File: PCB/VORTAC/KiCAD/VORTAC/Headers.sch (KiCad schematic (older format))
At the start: 15 parts, among them J1 MillMax_004, J10 HEATER, J11 STEPPER, J12 IO, J13 918-418K2023S40001, J2 MillMax_004, J3 DOCK, J4 USB_HOST, J5 FAN_01, J6 FAN_02, J7 LED, J8 HOTEND, J9 THERM

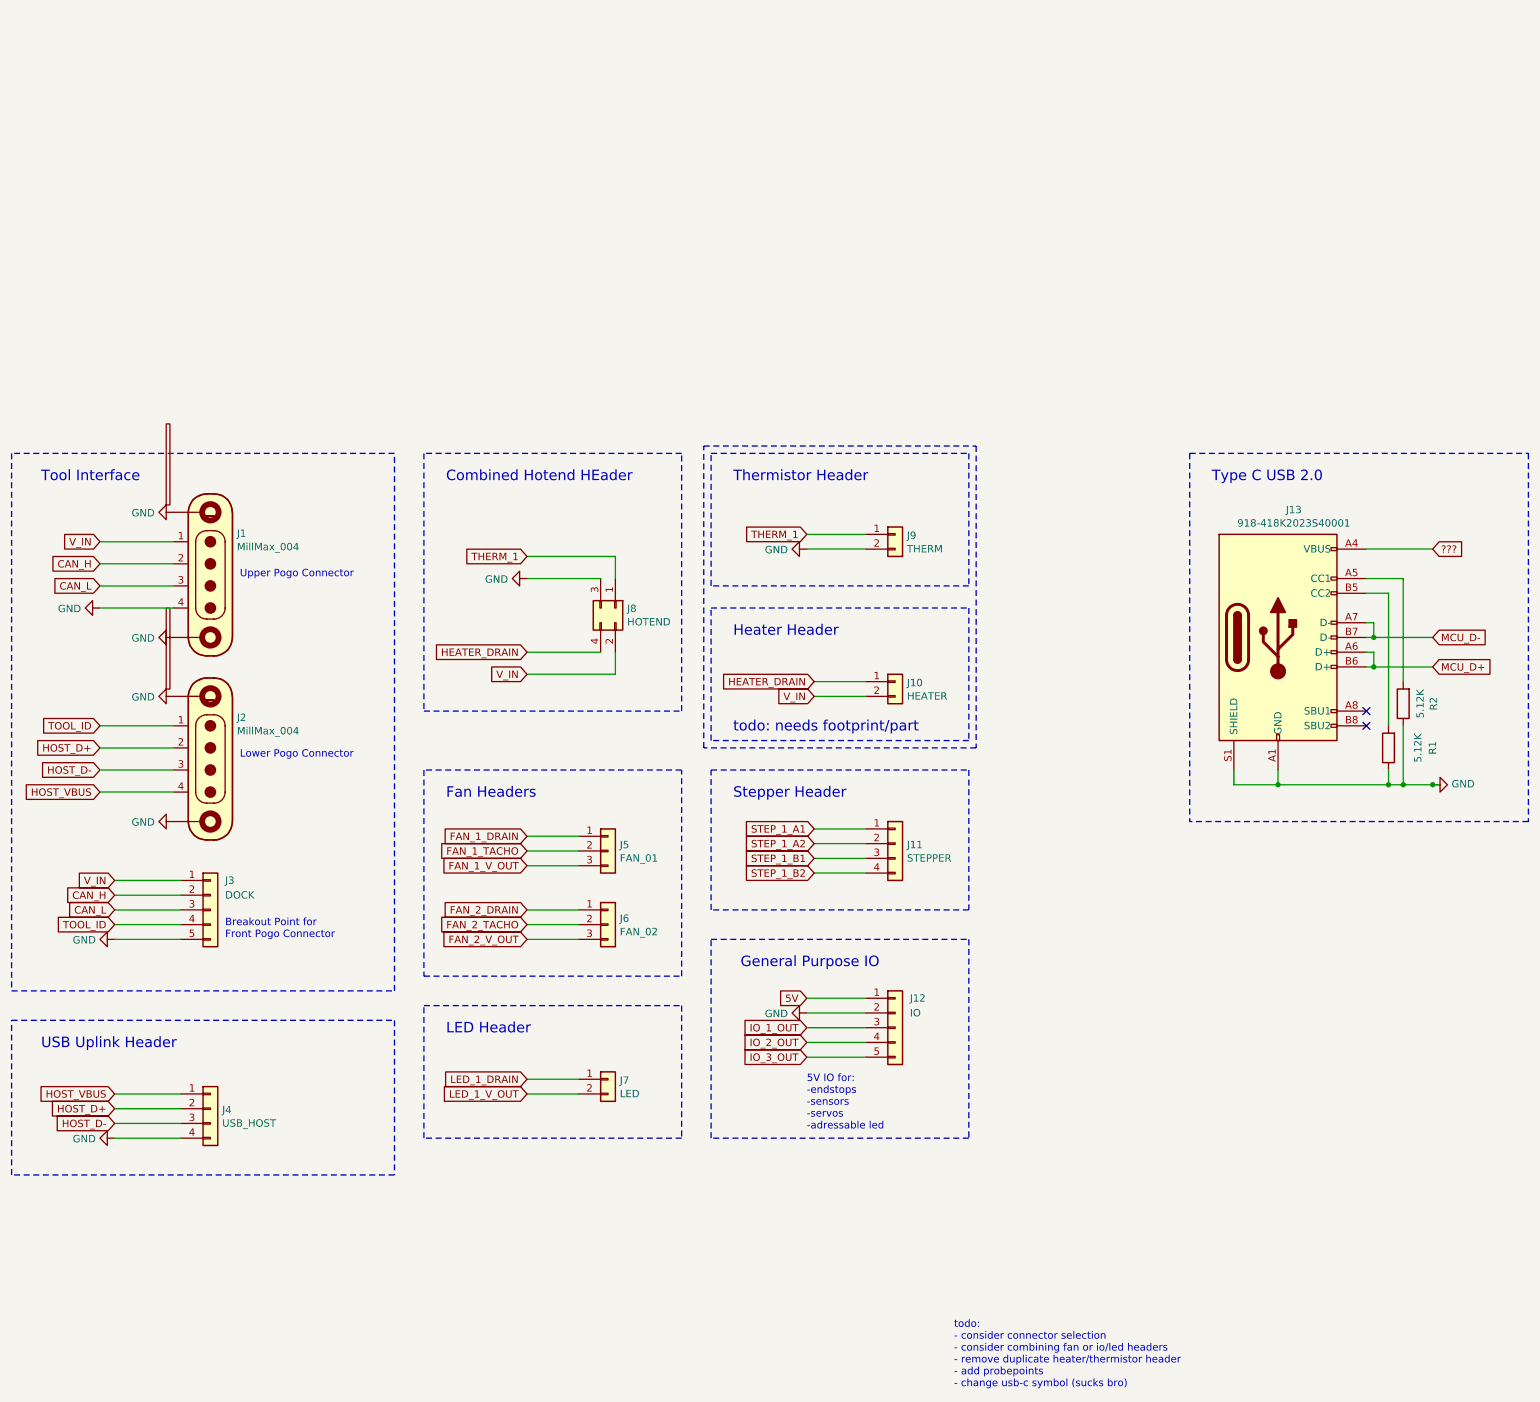
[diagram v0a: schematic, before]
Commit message: Auto stash before merge of "main" and "origin/main"
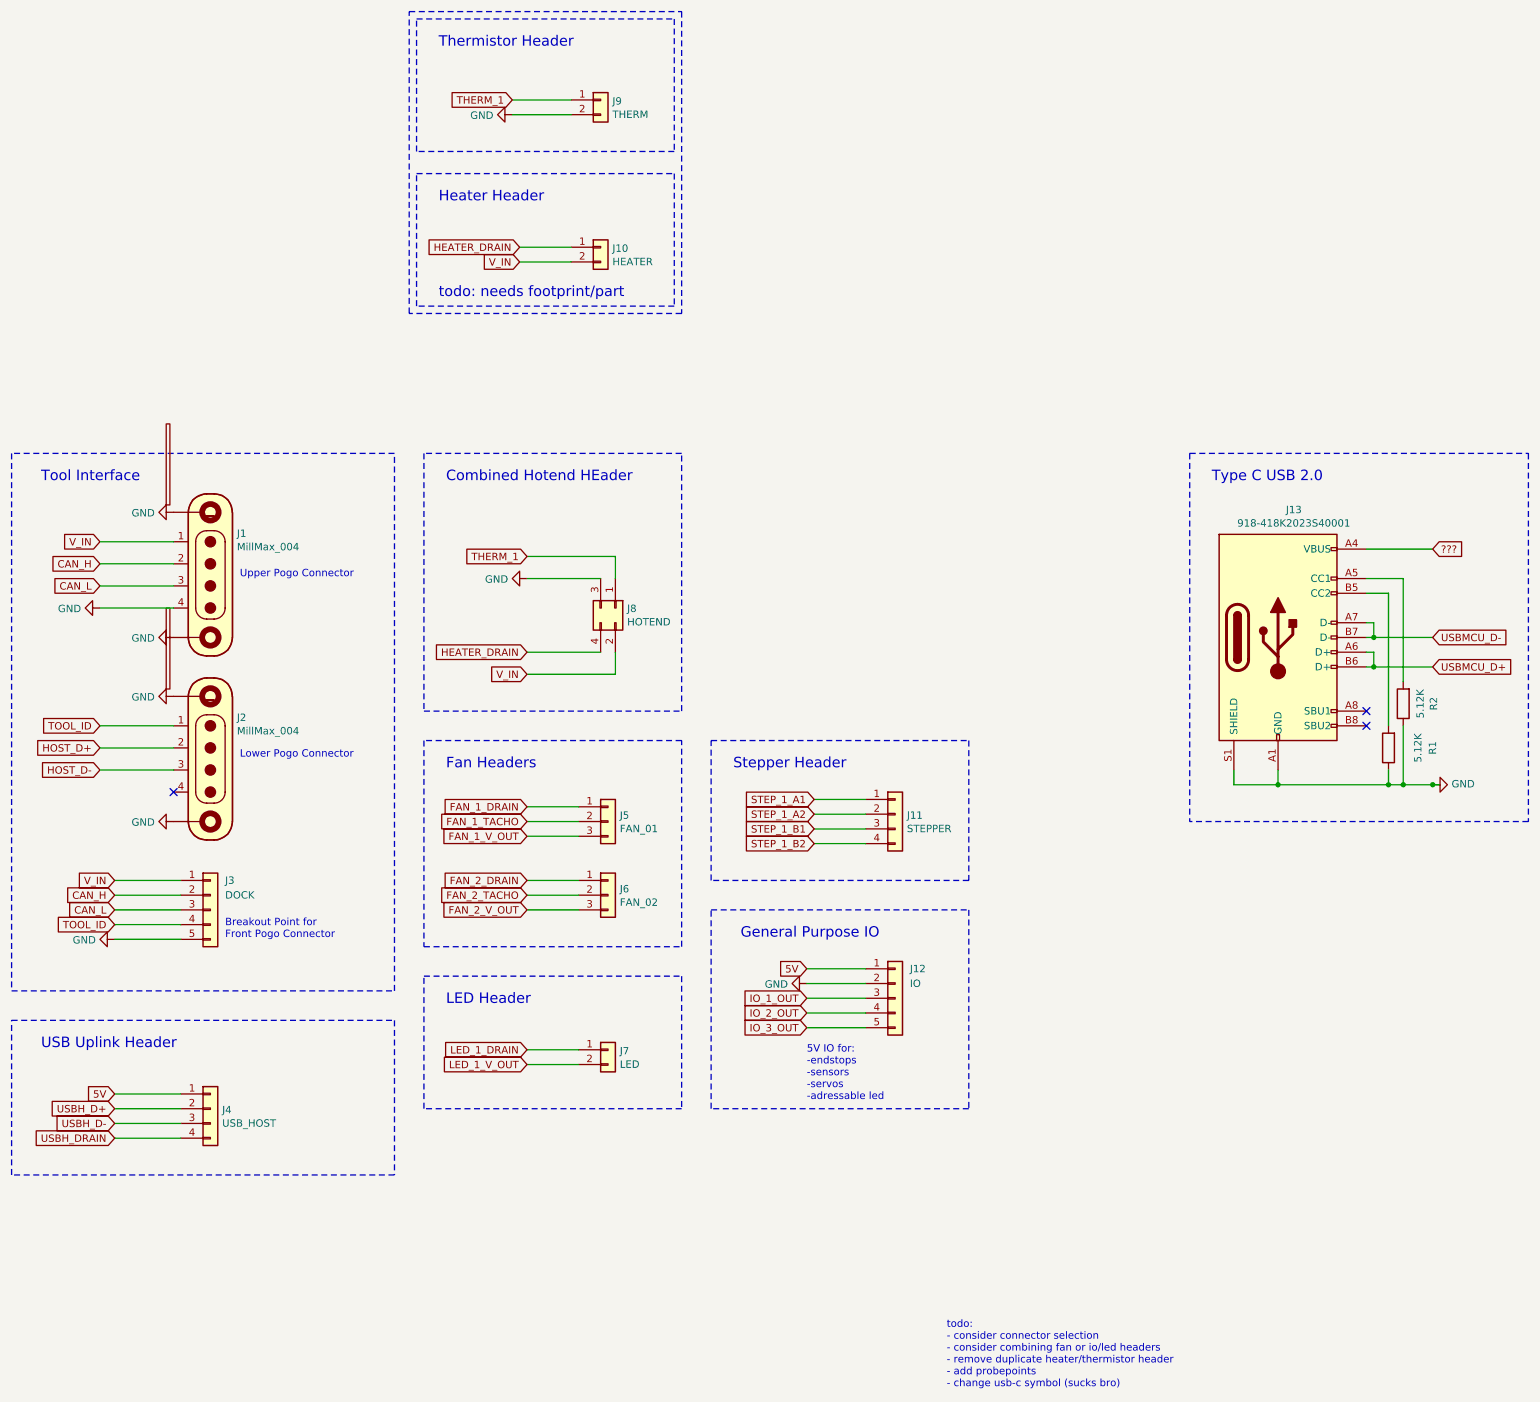
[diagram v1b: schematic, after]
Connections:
- net 5V: now also J4.1 (Pin_1)
- net GND: no longer J4.4 (Pin_4)
- net HOST_D+: no longer J4.2 (Pin_2)
- net HOST_D-: no longer J4.3 (Pin_3)
- net HOST_VBUS: no longer names the net of J2.4
- net HOST_VBUS: no longer J4.1 (Pin_1)
- net MCU_D+ renamed USBMCU_D+
- net MCU_D- renamed USBMCU_D-
- new net USBH_D+: J4.2 (Pin_2)
- new net USBH_D-: J4.3 (Pin_3)
- new net USBH_DRAIN: J4.4 (Pin_4)
- no-connect marks 2 -> 3
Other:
- moved on the sheet: J10, J11, J12, J5, J6, J7, J9
